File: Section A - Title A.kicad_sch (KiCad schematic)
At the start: 37 parts, among them Q1 SI2303CDS-T1-GE3, U1 AD7190WBRUZ, Y2 CSTCR4M91G53-R0

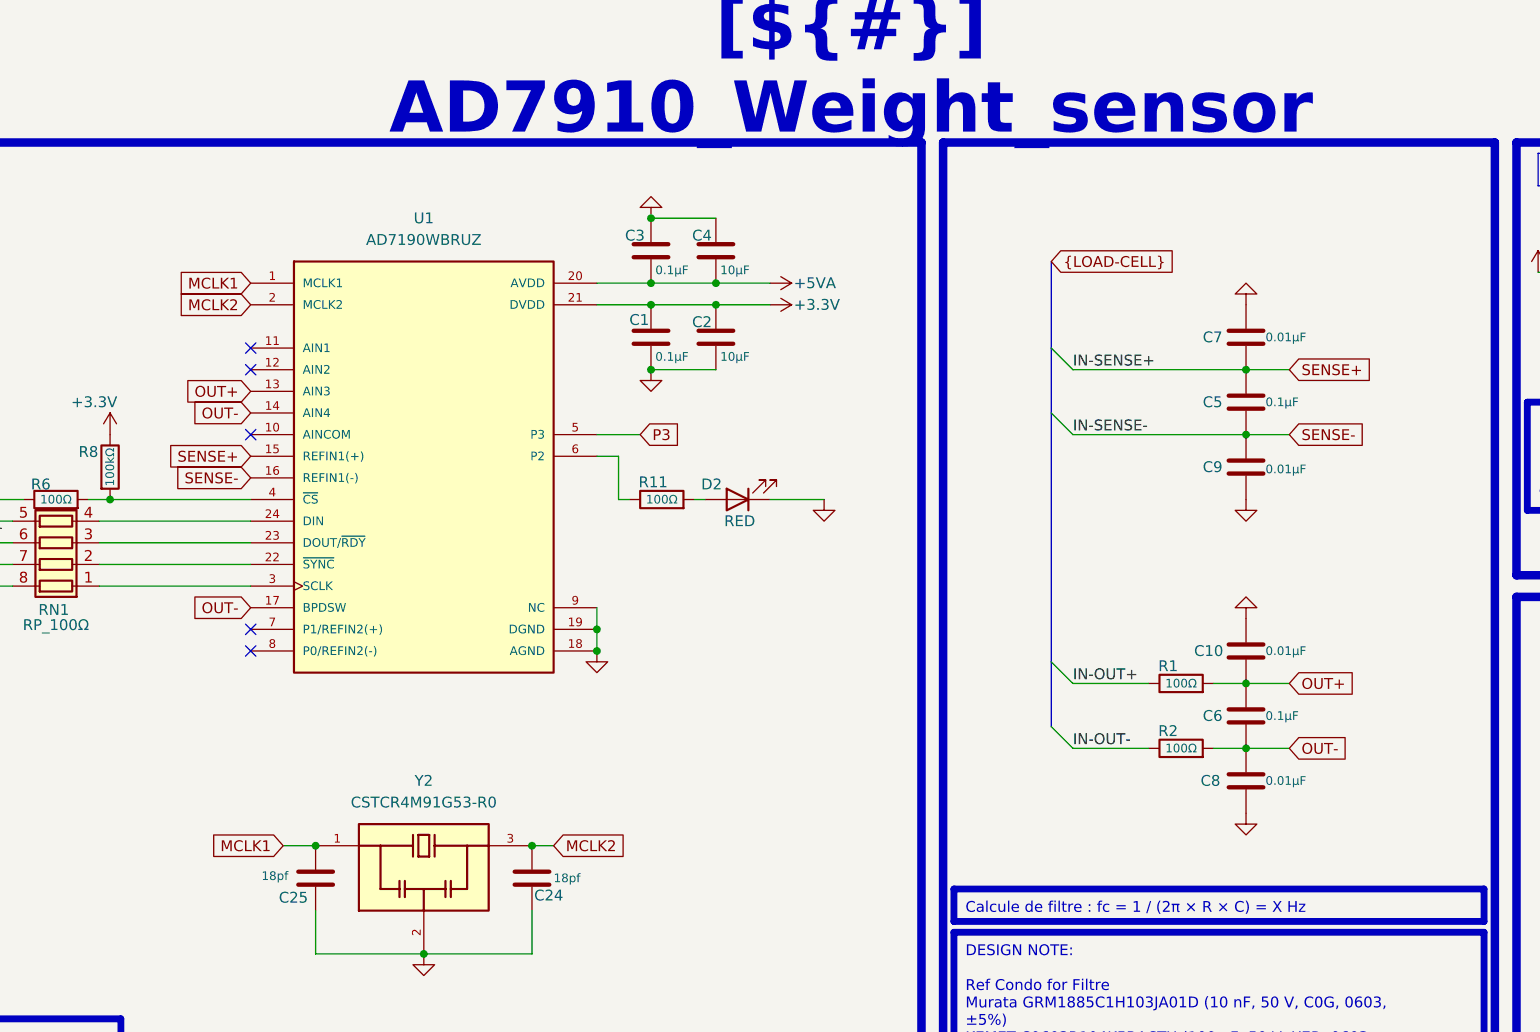
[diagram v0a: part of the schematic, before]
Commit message: Save KiCad 10 design work (schematic + PCB) since March
Co-Authored-By: Claude Opus 5.5 <noreply@anthropic.com>
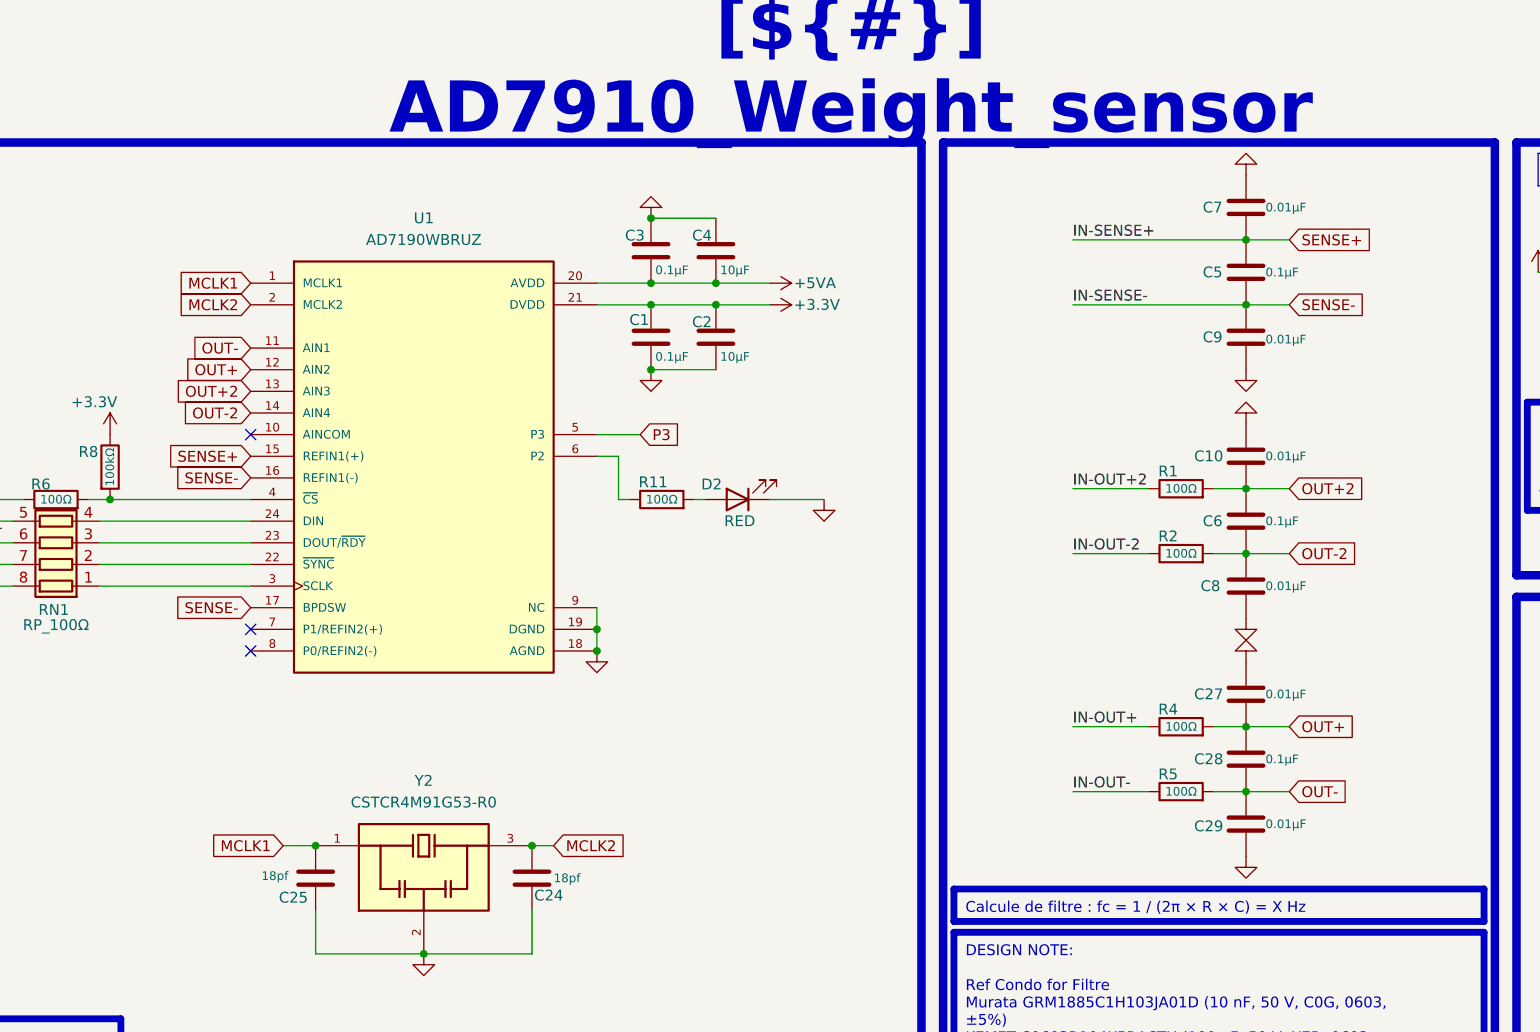
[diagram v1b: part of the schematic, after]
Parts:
- added C27, C29: 0.01µF, Capacitor_SMD:C_0603_1608Metric, symbol Device:C
- added C28: 0.1µF, Capacitor_SMD:C_0603_1608Metric, symbol Device:C
- added R4, R5: 100Ω, Resistor_SMD:R_0603_1608Metric, symbol Device:R
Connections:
- net GND: now also C27.1, C29.2
- net IN-OUT+: now also R4.1; no longer R1.1
- net IN-OUT-: now also R5.1; no longer R2.1
- net OUT+: now also U1.12 (AIN2), C27.2, C28.1, R4.2; no longer C10.2, C6.1, R1.2, U1.13 (AIN3)
- net OUT-: now also U1.11 (AIN1), C28.2, C29.1, R5.2; no longer C6.2, C8.1, R2.2, U1.14 (AIN4), U1.17 (BPDSW)
- net SENSE-: now also U1.17 (BPDSW)
- new net IN-OUT+2: R1.1
- new net IN-OUT-2: R2.1
- new net OUT+2: C10.2, C6.1, R1.2, U1.13 (AIN3)
- new net OUT-2: C6.2, C8.1, R2.2, U1.14 (AIN4)
- no-connect marks 5 -> 3
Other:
- moved on the sheet: C10, C5, C6, C7, C8, C9, R1, R2
